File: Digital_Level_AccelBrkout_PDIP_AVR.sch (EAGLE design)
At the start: 31 parts, among them CN1 Batt1, U1 NCP1402, U2 TPS79328DBVR, U3 ATMEGA328P-PU, U4 CD74HC4067, U5 NCP1402, Y1 16MHz

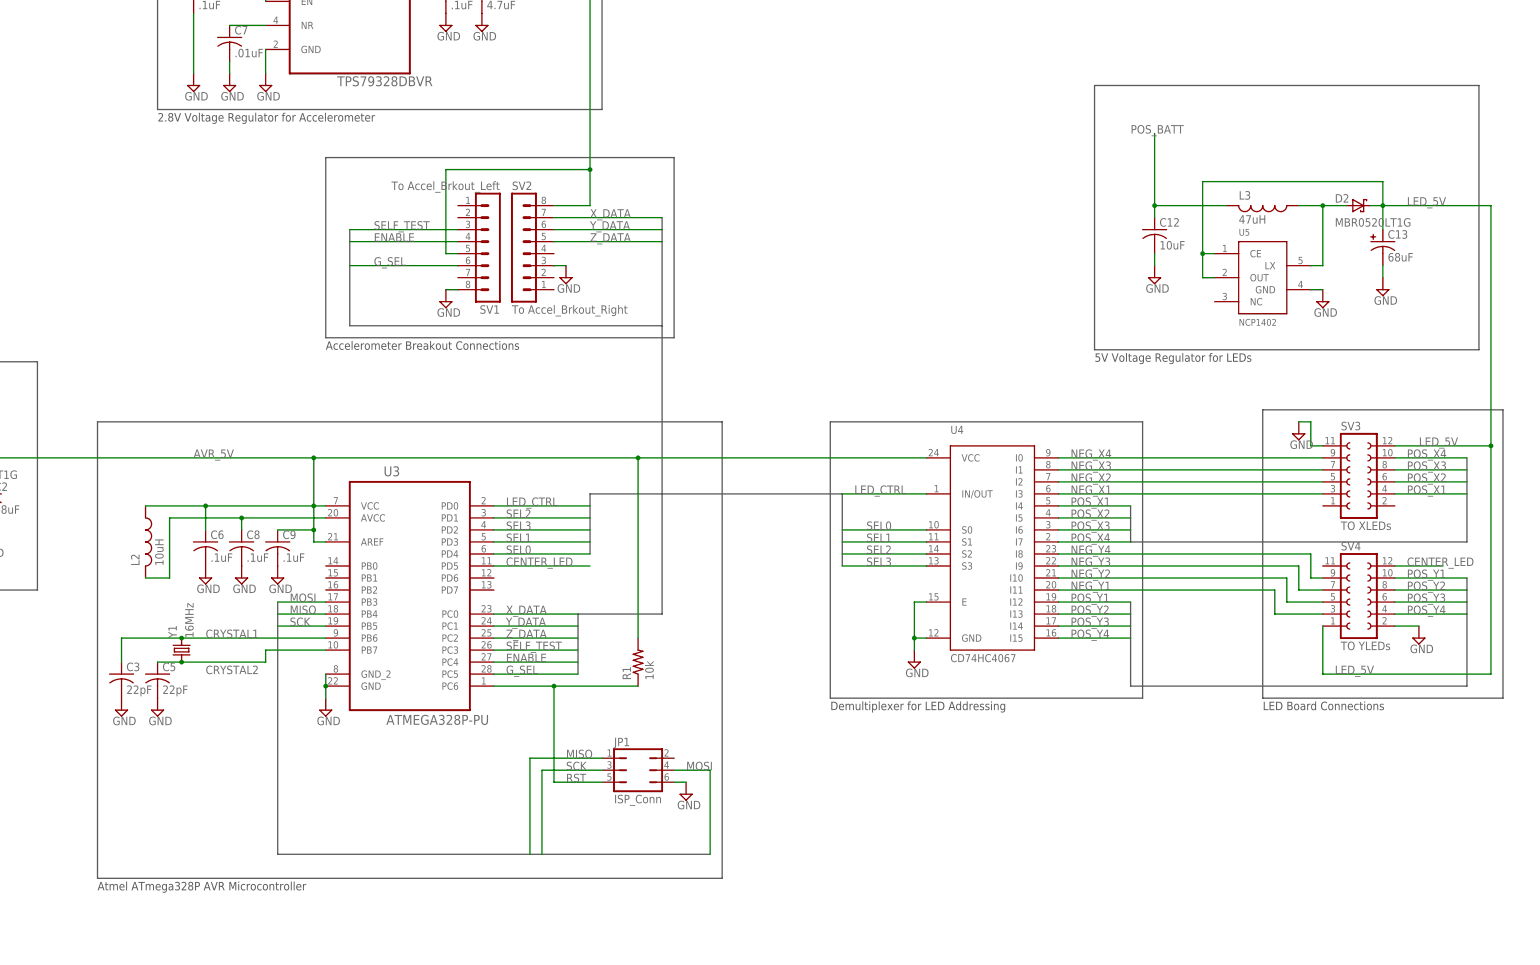
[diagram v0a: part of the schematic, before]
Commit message: Updated Schematic
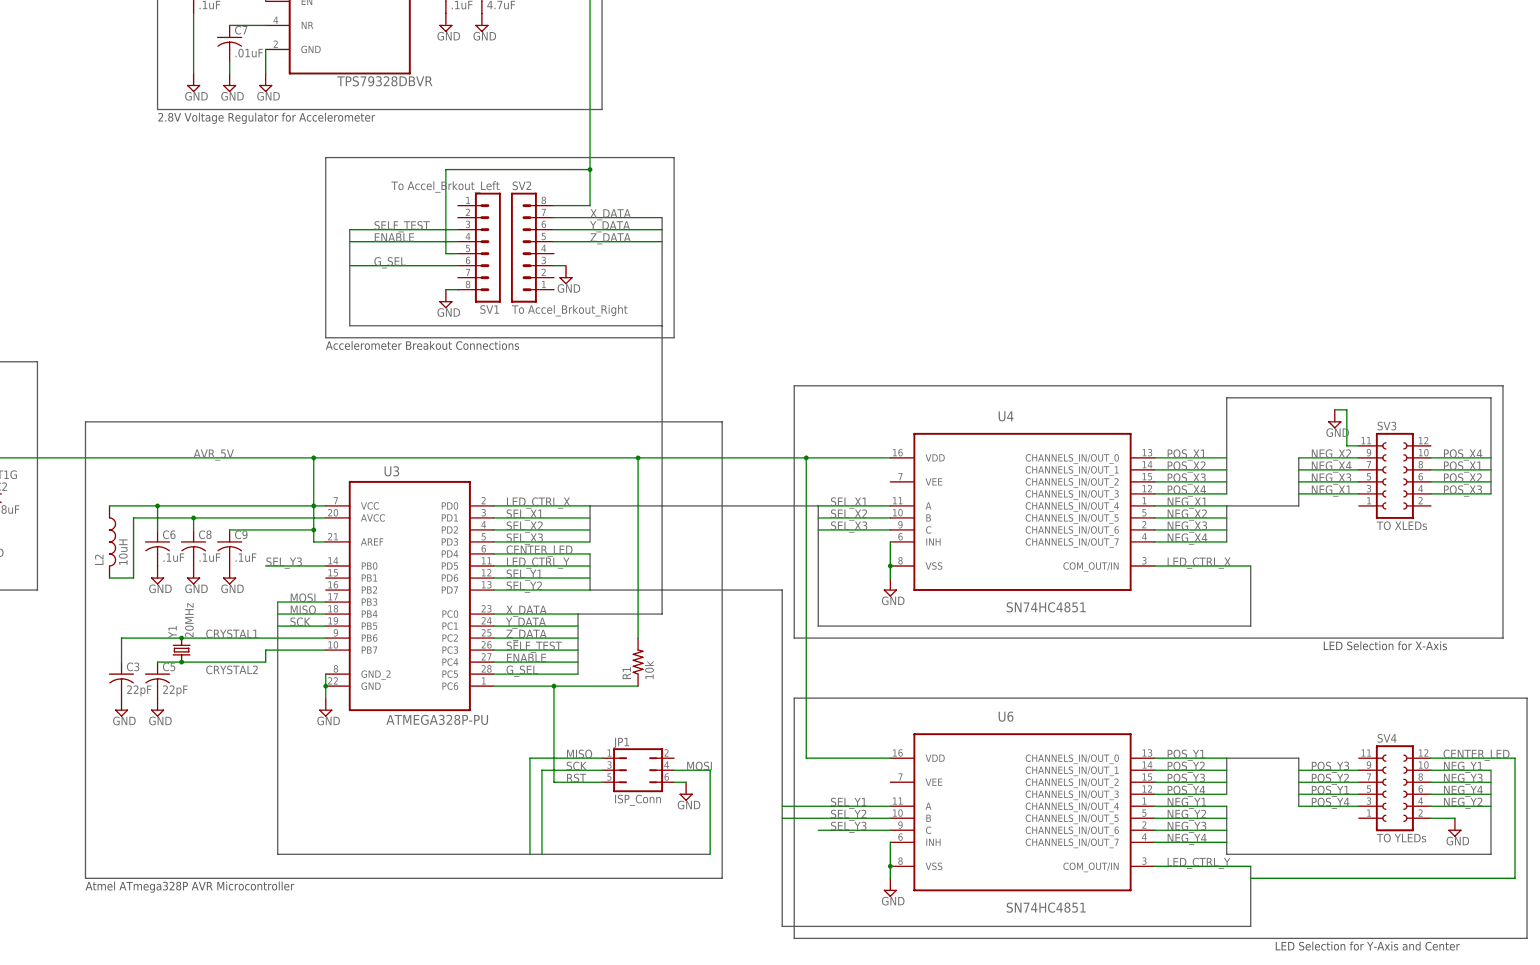
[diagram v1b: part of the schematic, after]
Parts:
- removed C12: 10uF, rcl:C-USC0805K
- removed C13: 68uF, cal_zabel:TANT_CAP
- removed D2: MBR0520LT1G, cal_zabel:ONSEMI_SCHOTTKY
- removed L3: 47uH, cal_zabel:BOURNS_INDUCTOR
- removed U5: NCP1402, cal_zabel:NCP1402
- added U6: SN74HC4851, Texas Instruments_By_element14_Batch_1:CD4051BE
- U4: value CD74HC4067 -> SN74HC4851; device cal_zabel:CD74HC4067 -> Texas Instruments_By_element14_Batch_1:CD4051BE
- Y1: value 16MHz -> 20MHz
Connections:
- removed net 5V_REG2_LX: D2.A, L3.1, U5.LX
- removed net LED_5V: C13.1, D2.K, SV3.12, SV4.1, U5.CE, U5.OUT
- removed net LED_CTRL: U3.PD0, U4.IN/OUT
- removed net SEL0: U3.PD4, U4.S0
- removed net SEL1: U3.PD3, U4.S1
- removed net SEL2: U3.PD1, U4.S2
- removed net SEL3: U3.PD2, U4.S3
- new net LED_CTRL_X: U3.PD0, U4.COM_OUT/IN
- new net LED_CTRL_Y: U3.PD5, U6.COM_OUT/IN
- new net SEL_X1: U3.PD1, U4.A
- new net SEL_X2: U3.PD2, U4.B
- new net SEL_X3: U3.PD3, U4.C
- new net SEL_Y1: U3.PD6, U6.A
- new net SEL_Y2: U3.PD7, U6.B
- new net SEL_Y3: U3.PB0, U6.C
- net AVR_5V: now also U4.VDD, U6.VDD; no longer U4.VCC
- net CENTER_LED: now also U3.PD4; no longer U3.PD5
- net GND: now also U4.INH, U4.VSS, U6.INH, U6.VSS; no longer C12.2, C13.2, U4.E, U4.GND, U5.GND
- net NEG_X1: now also U4.CHANNELS_IN/OUT_4; no longer U4.I3
- net NEG_X2: now also SV3.9, U4.CHANNELS_IN/OUT_5; no longer SV3.5, U4.I2
- net NEG_X3: now also SV3.5, U4.CHANNELS_IN/OUT_6; no longer SV3.7, U4.I1
- net NEG_X4: now also SV3.7, U4.CHANNELS_IN/OUT_7; no longer SV3.9, U4.I0
- net NEG_Y1: now also SV4.10, U6.CHANNELS_IN/OUT_4; no longer SV4.3, U4.I11
- net NEG_Y2: now also SV4.4, U6.CHANNELS_IN/OUT_5; no longer SV4.5, U4.I10
- net NEG_Y3: now also SV4.8, U6.CHANNELS_IN/OUT_6; no longer SV4.7, U4.I9
- net NEG_Y4: now also SV4.6, U6.CHANNELS_IN/OUT_7; no longer SV4.9, U4.I8
- net POS_BATT: no longer C12.1, L3.2
- net POS_X1: now also SV3.8, U4.CHANNELS_IN/OUT_0; no longer SV3.4, U4.I4
- net POS_X2: now also U4.CHANNELS_IN/OUT_1; no longer U4.I5
- net POS_X3: now also SV3.4, U4.CHANNELS_IN/OUT_2; no longer SV3.8, U4.I6
- net POS_X4: now also U4.CHANNELS_IN/OUT_3; no longer U4.I7
- net POS_Y1: now also SV4.5, U6.CHANNELS_IN/OUT_0; no longer SV4.10, U4.I12
- net POS_Y2: now also SV4.7, U6.CHANNELS_IN/OUT_1; no longer SV4.8, U4.I13
- net POS_Y3: now also SV4.9, U6.CHANNELS_IN/OUT_2; no longer SV4.6, U4.I14
- net POS_Y4: now also SV4.3, U6.CHANNELS_IN/OUT_3; no longer SV4.4, U4.I15
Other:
- note added: "LED Selection for X-Axis"
- note added: "LED Selection for Y-Axis and Center"
- note removed: "5V Voltage Regulator for LEDs"
- note removed: "Demultiplexer for LED Addressing"
- note removed: "LED Board Connections"
- moved on the sheet: C6, C8, C9, L2, SV3, SV4
